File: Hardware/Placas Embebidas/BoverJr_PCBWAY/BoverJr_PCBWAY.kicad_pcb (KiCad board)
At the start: 2 copper layers, 100 x 100.1 mm, 47 parts, among them J1 Encoder Derecho, J10 7.4v, J11 Cable_PAD, J2 Encoder Izquierdo, J3 Programador, J4 Distancia_Der, J5 Distancia_Izq, J6 Cable_PAD, J7 Cable_PAD, J8 Distancia_Frontal, J9 Cable_PAD, SW1 SW_SPDT, U1 ESP32-WROOM-32E, U2 MPU, U3 AMS1117-5.0, U5 DRV8833, U7 AMS1117-3.3

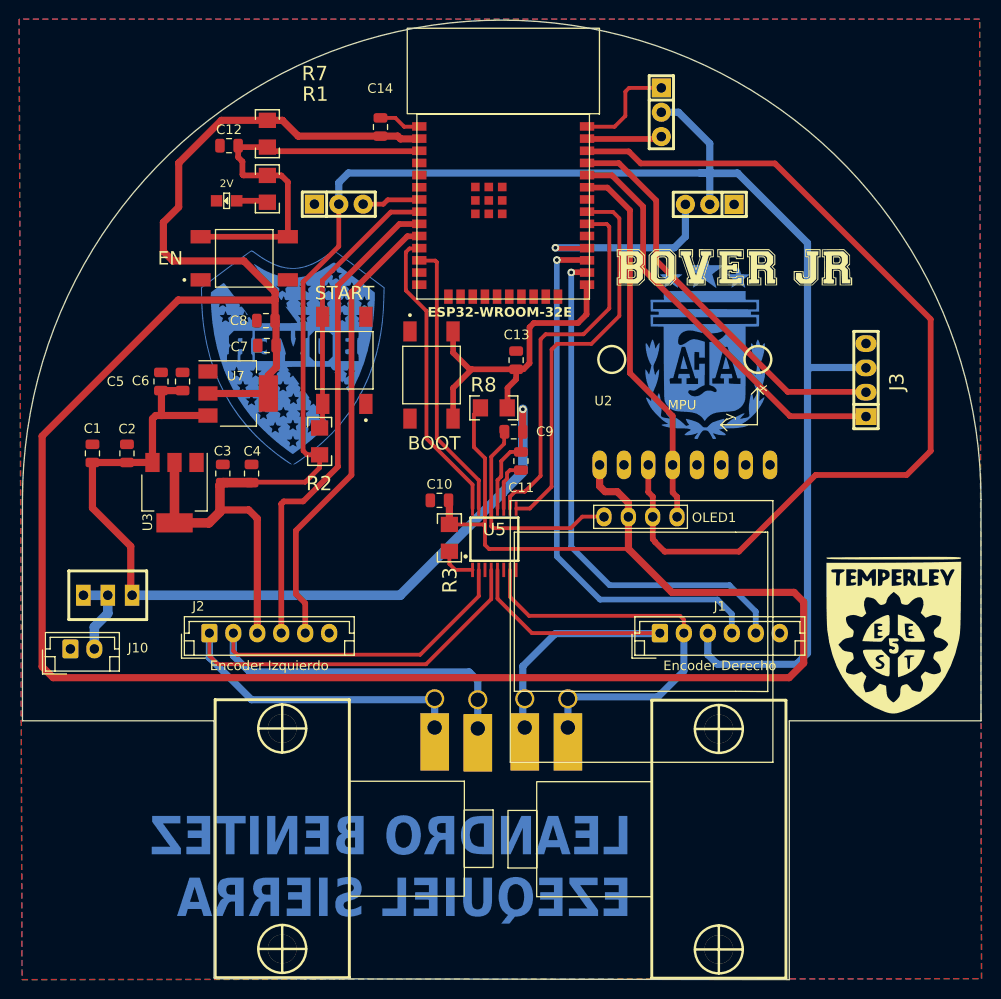
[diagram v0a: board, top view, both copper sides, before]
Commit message: soy un boludo
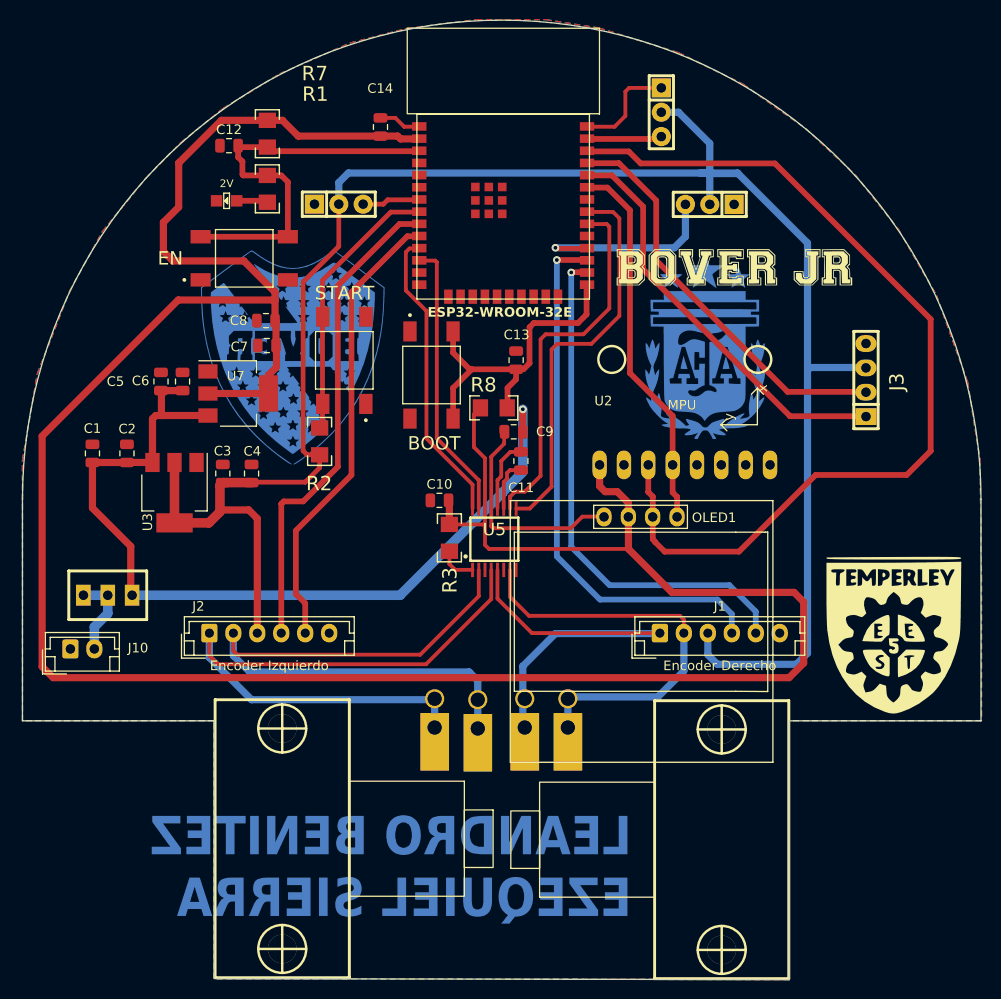
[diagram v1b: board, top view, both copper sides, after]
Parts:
- moved H2 0.30 mm to (172.9, 115.3)
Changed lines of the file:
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@@
   )
   (footprint "EESTN5:Pololu_Micro_Con_Soporte_Simple" (layer "F.Cu")
-    (at 172.65 115.25 90)
+    (at 172.95 115.3 90)
     (descr "Pololu Micro Gear Motor W/Mount")
     (property "Sheetfile" "BoverJr_PCBWAY.kicad_sch")
@@
     (pad "3" thru_hole rect (at 2.54 0) (size 1.524 2.19964) (drill 1.00076) (layers "*.Cu" "*.Mask" "F.SilkS")
       (net 15 "VCC") (pinfunction "C") (pintype "passive"))
-    (model "SW-SPDT-TH-100Mils-Vertical.wrl"
+    (model "C:/Users/juana/Dropbox/GIT/Librerias-Kicad/EESTN5.3dshapes/SW-SPDT-TH-100Mils-Vertical.wrl"
       (offset (xyz 0 0 0))
       (scale (xyz 1 1 1))
@@
     (polygon
       (pts
-        (xy 200.055689 129.799902)
-        (xy 199.855689 29.699902)
-        (xy 99.655689 29.699902)
-        (xy 99.955689 129.899902)
+        (xy 180 129.9)
+        (xy 120 129.8)
+        (xy 120 102.9)
+        (xy 100 102.9)
+        (xy 100 75.7)
+        (xy 101.55 66.7)
+        (xy 104.9 58.1)
+        (xy 108.35 51.85)
+        (xy 112.9 46.25)
+        (xy 116.55 42.55)
+        (xy 120.95 39)
+        (xy 126.85 35.4)
+        (xy 134.15 32.2)
+        (xy 140.15 30.655)
+        (xy 147.35 29.75)
+        (xy 154.6 29.75)
+        (xy 160.16 30.625)
+        (xy 168.45 33.2)
+        (xy 175.2 36.5)
+        (xy 181.7 41.1)
+        (xy 186.85 45.9)
+        (xy 191.4 51.65)
+        (xy 195.35 58.5)
+        (xy 198.6 67.55)
+        (xy 199.9 75.65)
+        (xy 200.05 87.8)
+        (xy 200.05 102.9)
+        (xy 180 102.9)
       )
     )
